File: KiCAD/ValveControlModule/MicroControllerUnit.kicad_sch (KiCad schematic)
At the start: 7 parts, among them U1 XIAO-RP2040-DIP

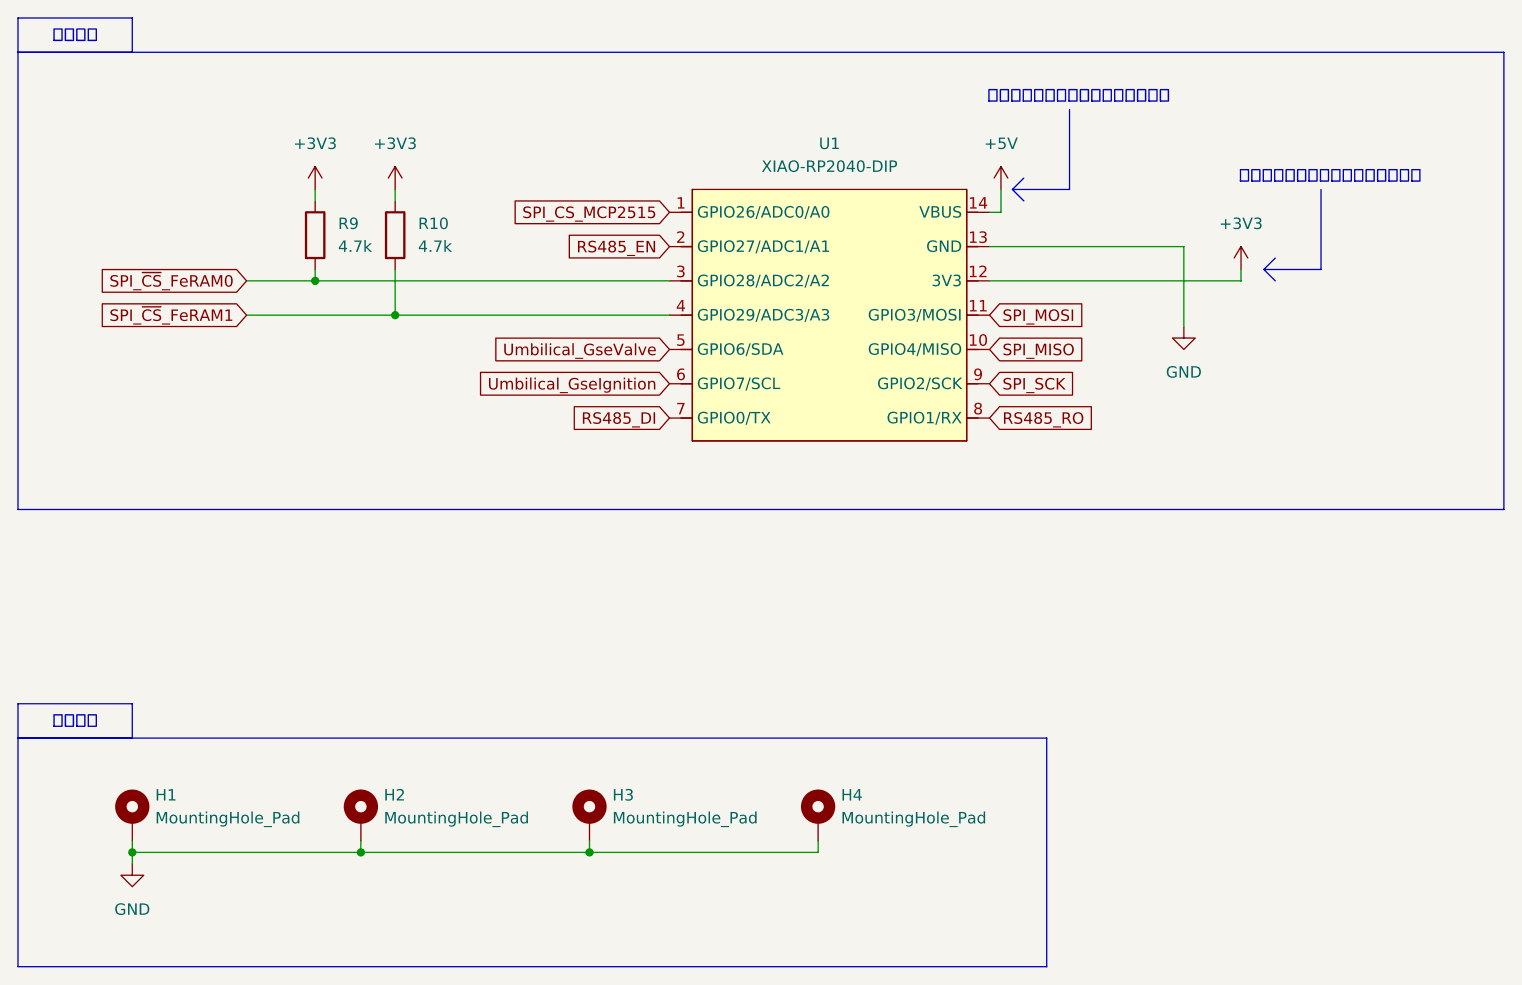
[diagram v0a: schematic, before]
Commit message: Build-2完成．発注．
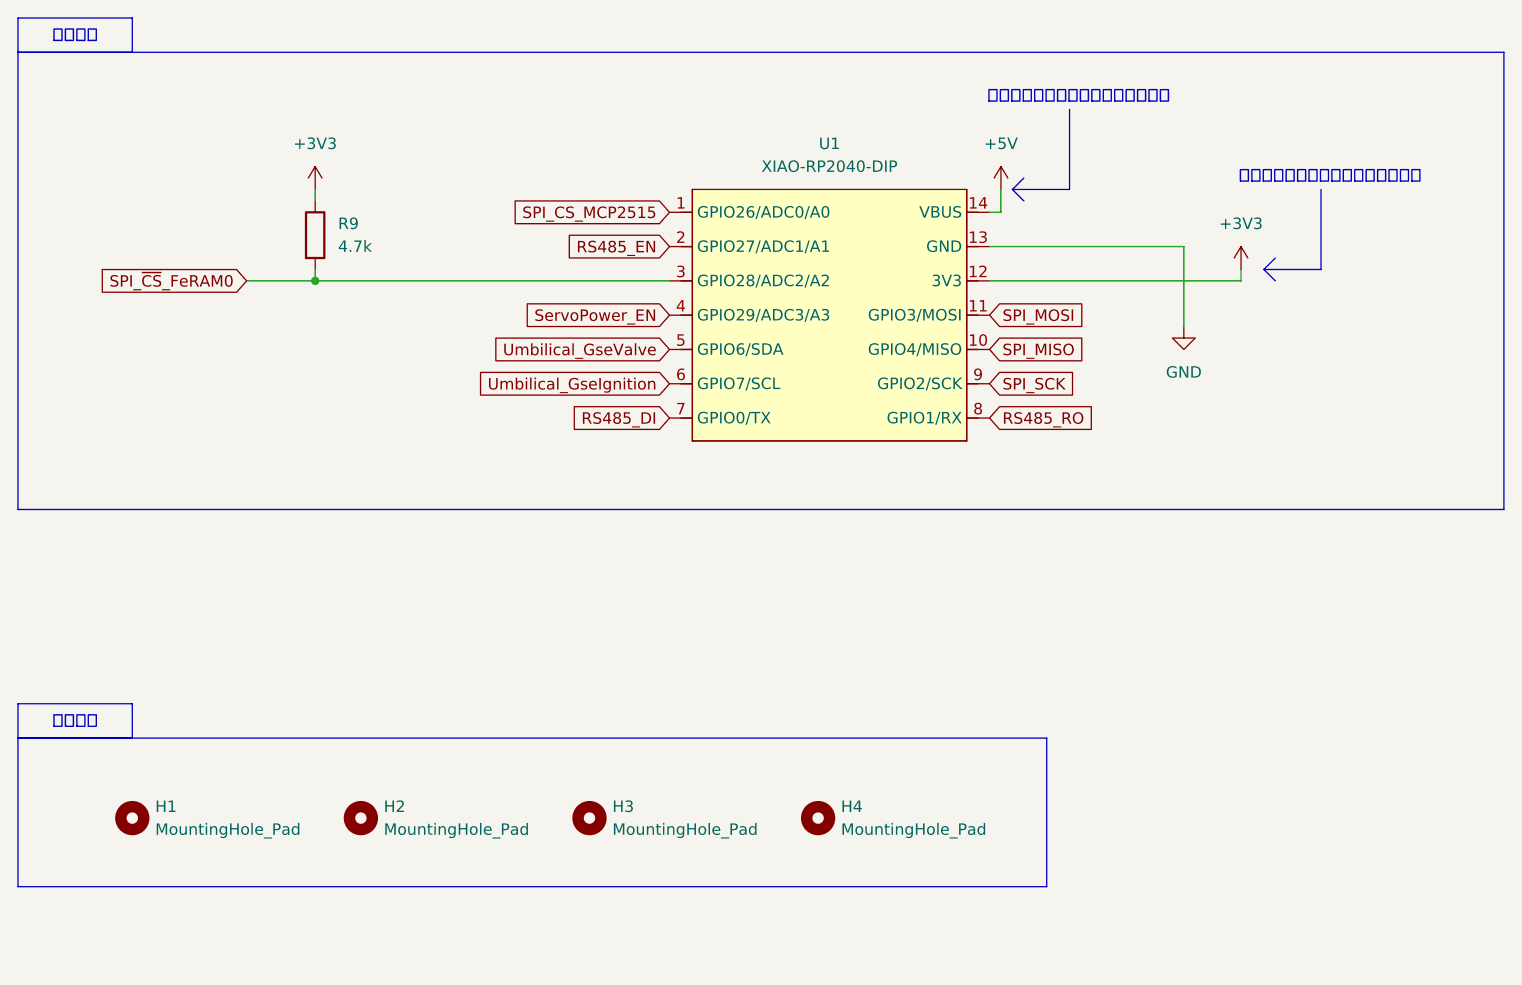
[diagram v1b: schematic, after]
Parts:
- removed R10: 4.7k, Resistor_SMD:R_0603_1608Metric_Pad0.98x0.95mm_HandSolder, symbol Device:R
- H1, H2, H3, H4: symbol Mechanical:MountingHole_Pad -> Mechanical:MountingHole; now in the parts list
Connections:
- net GND: no longer H1.1, H2.1, H3.1, H4.1
- net SPI_~{CS}_FeRAM1 renamed ServoPower_EN
